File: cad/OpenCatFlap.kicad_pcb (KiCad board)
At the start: 2 copper layers, 97 x 53 mm, 17 parts, among them P1 Outside PIR, P2 IR Barrier Outside, P3 IR Barrier Inside, P4 Servo Outside, P5 Servo Inside, P6 RFID inside, P7 RFID outside, U1 DOIT-ESP32-DEVKIT-V1, U2 AMN33111, U3 5V

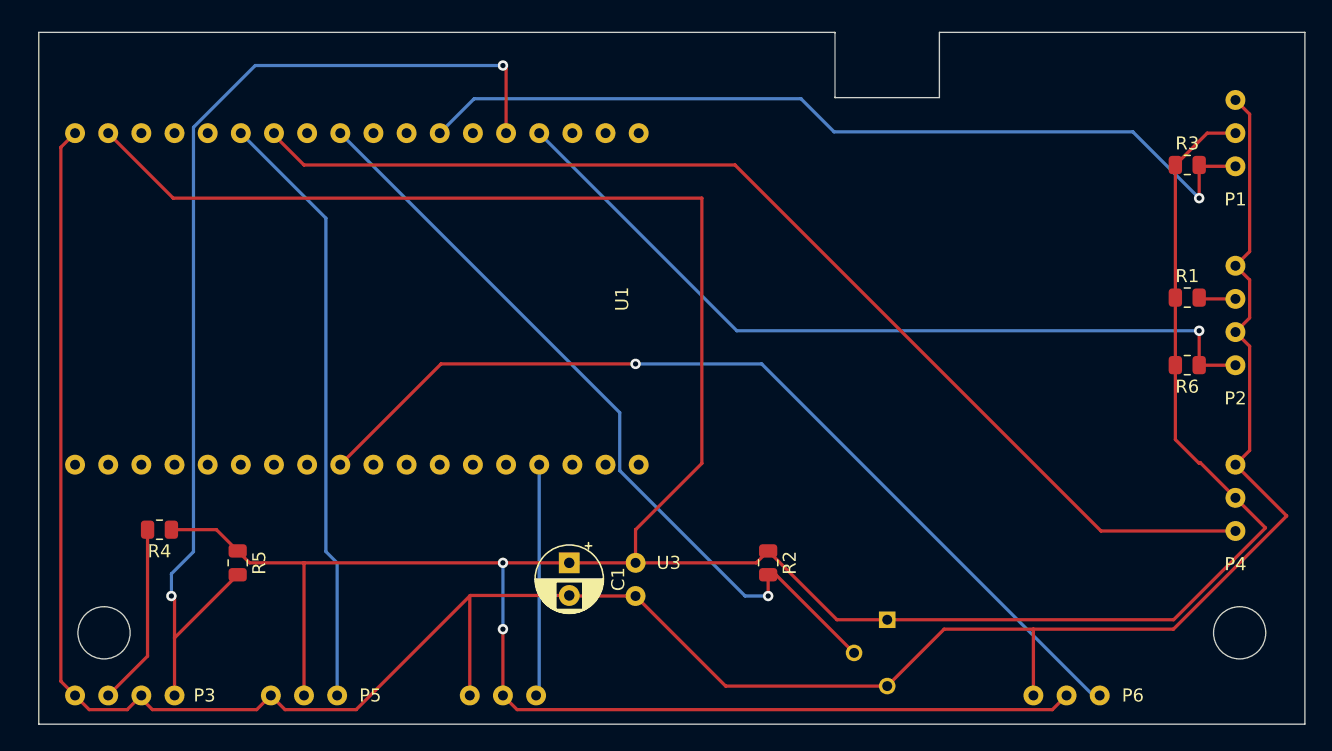
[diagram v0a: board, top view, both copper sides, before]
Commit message: boop
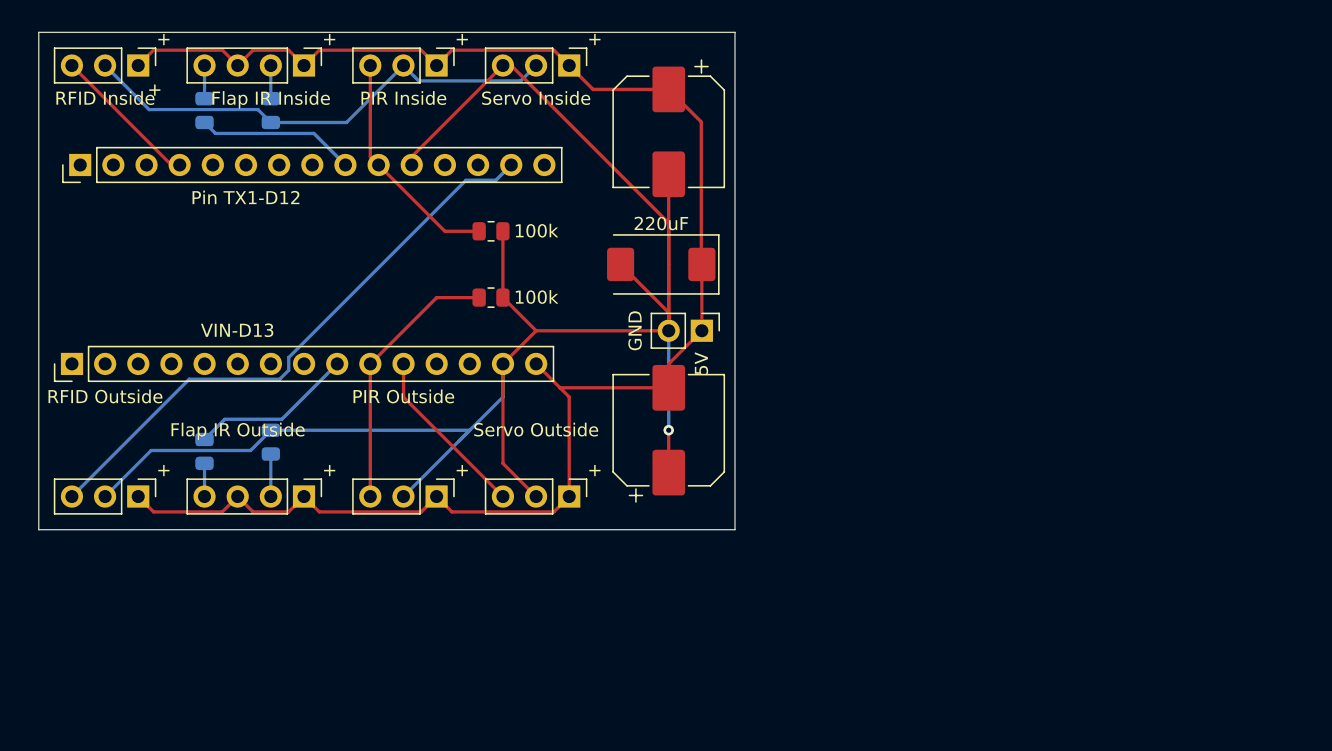
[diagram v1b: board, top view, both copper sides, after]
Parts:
- removed C1: 220uF, Capacitor_THT:CP_Radial_D5.0mm_P2.50mm
- removed R6: 100R, Resistor_SMD:R_0805_2012Metric
- removed U1: DOIT-ESP32-DEVKIT-V1, OpenCatFlap:ESP32-DOIT-DEVKIT
- removed U2: AMN33111, OpenCatFlap:AMN33111_PAN
- added ArduinoESP32_L1: VIN-D13, Connector_PinHeader_2.54mm:PinHeader_1x15_P2.54mm_Vertical, F.Cu at (93.7, 83.7)
- added ArduinoESP32_R1: Pin TX1-D12, Connector_PinHeader_2.54mm:PinHeader_1x15_P2.54mm_Vertical, F.Cu at (94.4, 68.5)
- added C2: C_Polarized, Capacitor_SMD:CP_Elec_8x10, F.Cu at (139.5, 65.9)
- added C3: C_Polarized, Capacitor_SMD:CP_Elec_8x10, F.Cu at (139.5, 88.8)
- added C4: 220uF, Capacitor_Tantalum_SMD:CP_EIA-7343-43_Kemet-X, F.Cu at (138.9, 76.1)
- added P8: PIR Inside, Connector_PinHeader_2.54mm:PinHeader_1x03_P2.54mm_Vertical, F.Cu at (121.7, 60.9)
- added R7: 100k, Resistor_SMD:R_0805_2012Metric, F.Cu at (125.8, 73.6)
- P1: value Outside PIR -> PIR Outside; footprint OpenCatFlap:PIR Header -> Connector_PinHeader_2.54mm:PinHeader_1x03_P2.54mm_Vertical
- P2: value IR Barrier Outside -> Flap IR Outside; footprint OpenCatFlap:IR Barrier Header -> Connector_PinHeader_2.54mm:PinHeader_1x04_P2.54mm_Vertical
- P3: value IR Barrier Inside -> Flap IR Inside; footprint OpenCatFlap:IR Barrier Header -> Connector_PinHeader_2.54mm:PinHeader_1x04_P2.54mm_Vertical
- P4, P5: footprint OpenCatFlap:Servo Header -> Connector_PinHeader_2.54mm:PinHeader_1x03_P2.54mm_Vertical
- P6: value RFID inside -> RFID Inside; footprint OpenCatFlap:PIR Header -> Connector_PinHeader_2.54mm:PinHeader_1x03_P2.54mm_Vertical
- P7: value RFID outside -> RFID Outside; footprint OpenCatFlap:PIR Header -> Connector_PinHeader_2.54mm:PinHeader_1x03_P2.54mm_Vertical
- R1, R4, R5: moved to B.Cu
- R3: value 100k -> 100R; moved to B.Cu
- U3: footprint OpenCatFlap:Power Header -> Connector_PinHeader_2.54mm:PinHeader_1x02_P2.54mm_Vertical
- moved P6 92.4 mm to (98.8, 60.9), turned to -90 degrees
- moved R1 76.6 mm to (103.9, 64.3), turned to -90 degrees
- moved P2 73.5 mm to (111.5, 93.9), turned to -90 degrees
- moved R3 73.3 mm to (109.0, 89.7), turned to 90 degrees
- moved P1 64.5 mm to (121.7, 93.9), turned to -90 degrees
- moved P5 53.4 mm to (131.8, 60.9), turned to -90 degrees
- moved P3 51.3 mm to (111.5, 60.9), turned to -90 degrees
- moved P4 51.1 mm to (131.8, 93.9), turned to -90 degrees
- moved P7 38.7 mm to (98.8, 93.9), turned to -90 degrees
- moved R4 33.2 mm to (109.0, 64.3), turned to 90 degrees
- moved R2 29.4 mm to (125.8, 78.6), turned to 180 degrees
- moved U3 20.9 mm to (142.0, 81.2), turned to -90 degrees
- moved R5 8.90 mm to (103.9, 90.4), turned to 90 degrees
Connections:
- net +5V renamed Net-(ArduinoESP32_L1-Pin_15)
- P1 pad 2: GND -> Net-(ArduinoESP32_L1-Pin_14)
- P1 pad 3: Net-(P1-In) -> Net-(ArduinoESP32_L1-Pin_10)
- P4 pad 2: GND -> Net-(ArduinoESP32_L1-Pin_14)
- P5 pad 2: GND -> Net-(ArduinoESP32_L1-Pin_14)
- P6 pad 2: GND -> Net-(ArduinoESP32_L1-Pin_14)
- P7 pad 2: GND -> Net-(ArduinoESP32_L1-Pin_14)
- R1 pad 1: GND -> Net-(P3-D-)
- R1 pad 2: Net-(P2-E-) -> Net-(ArduinoESP32_R1-Pin_9)
- R2 pad 1: GND -> Net-(ArduinoESP32_L1-Pin_14)
- R2 pad 2: Net-(U1-GPIO27_ADC2-CH7_RTC-GPIO17) -> Net-(ArduinoESP32_L1-Pin_10)
- R3 pad 1: GND -> Net-(P2-E-)
- R3 pad 2: Net-(P1-In) -> Net-(ArduinoESP32_L1-Pin_14)
- R4 pad 1: GND -> Net-(ArduinoESP32_L1-Pin_14)
- R5 pad 1: GND -> Net-(P2-D-)
- R5 pad 2: Net-(P3-D-) -> Net-(ArduinoESP32_L1-Pin_9)
- U3 pad 2: GND -> Net-(ArduinoESP32_L1-Pin_14)
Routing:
- net GND: track 268.8 -> 0.00 mm, vias 2 -> 0
- net Net-(ArduinoESP32_L1-Pin_14): track 0.00 -> 170.6 mm, vias 0 -> 1
- net Net-(P3-D-): track 82.1 -> 2.54 mm, vias 2 -> 0
- net Net-(ArduinoESP32_L1-Pin_15): track 200.4 -> 126.7 mm
- net Net-(ArduinoESP32_L1-Pin_11): track 86.6 -> 13.3 mm
- net Net-(P1-In): track 67.8 -> 0.00 mm, vias 1 -> 0
- net Net-(U1-GPIO27_ADC2-CH7_RTC-GPIO17): track 60.8 -> 0.00 mm, vias 1 -> 0
- net Net-(ArduinoESP32_R1-Pin_4): track 71.9 -> 12.0 mm, vias 1 -> 0
- net Net-(P2-D-): track 62.2 -> 2.54 mm, vias 1 -> 0
- net Net-(ArduinoESP32_R1-Pin_11): track 46.1 -> 10.5 mm
- net Net-(ArduinoESP32_R1-Pin_14): track 17.8 -> 44.7 mm
- net Net-(ArduinoESP32_L1-Pin_10): track 0.00 -> 20.6 mm
- net Net-(ArduinoESP32_R1-Pin_10): track 0.00 -> 17.7 mm
- net Net-(ArduinoESP32_L1-Pin_9): track 0.00 -> 12.6 mm
- net Net-(ArduinoESP32_R1-Pin_9): track 0.00 -> 12.1 mm
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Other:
- board size 97 x 53 mm -> 53.3 x 38.1 mm
- board text added: "+"
- board text added: "GND"
